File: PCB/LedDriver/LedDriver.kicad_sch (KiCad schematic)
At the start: 36 parts, among them J101 LCD, J102 Conn_01x07_Female, J103 Conn_01x02_Male, J104 Conn_01x02_Male, J105 Conn_01x02_Male, J106 Conn_01x02_Male, J107 DC+5V, J108 Conn_01x08_Male, J109 Conn_01x08_Male, J110 Conn_01x08_Male, J111 Conn_01x02_Male, SW101 SW_Push, SW102 SW_Push, SW103 SW_Push, SW104 SW_Push, SW105 SW_Push, SW106 SW_Push, SW107 SW_Push, U101 MW-R-WX, U102 LM1117-3.3, U103 LM35-LP

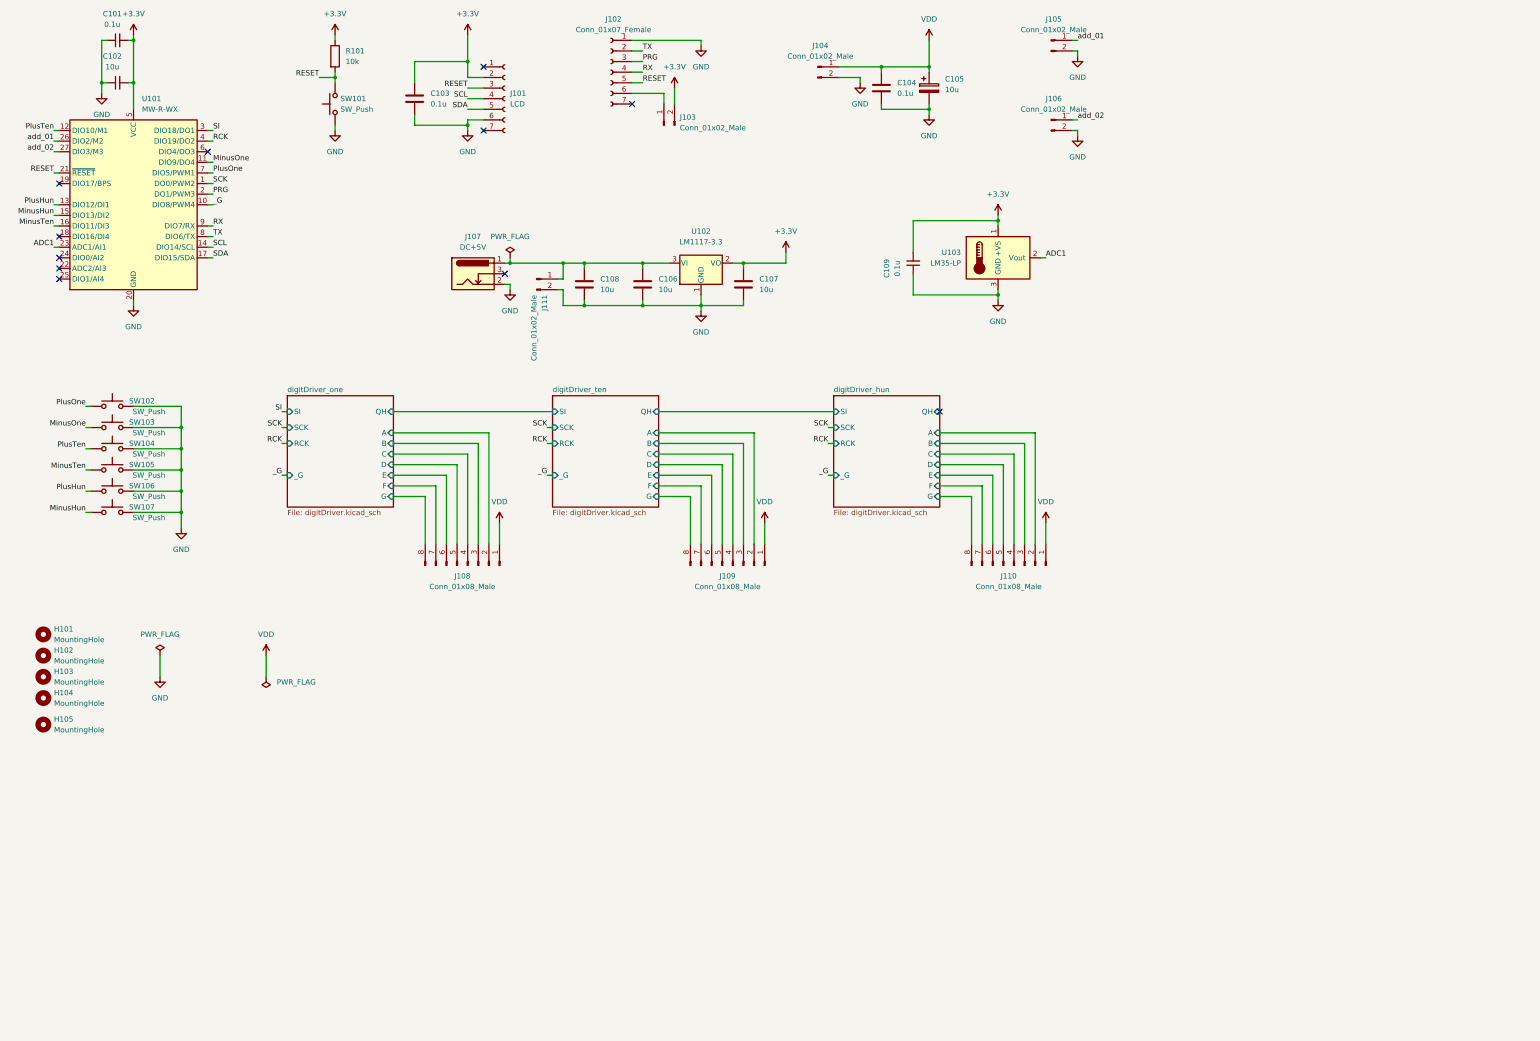
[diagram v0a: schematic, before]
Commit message: branch change
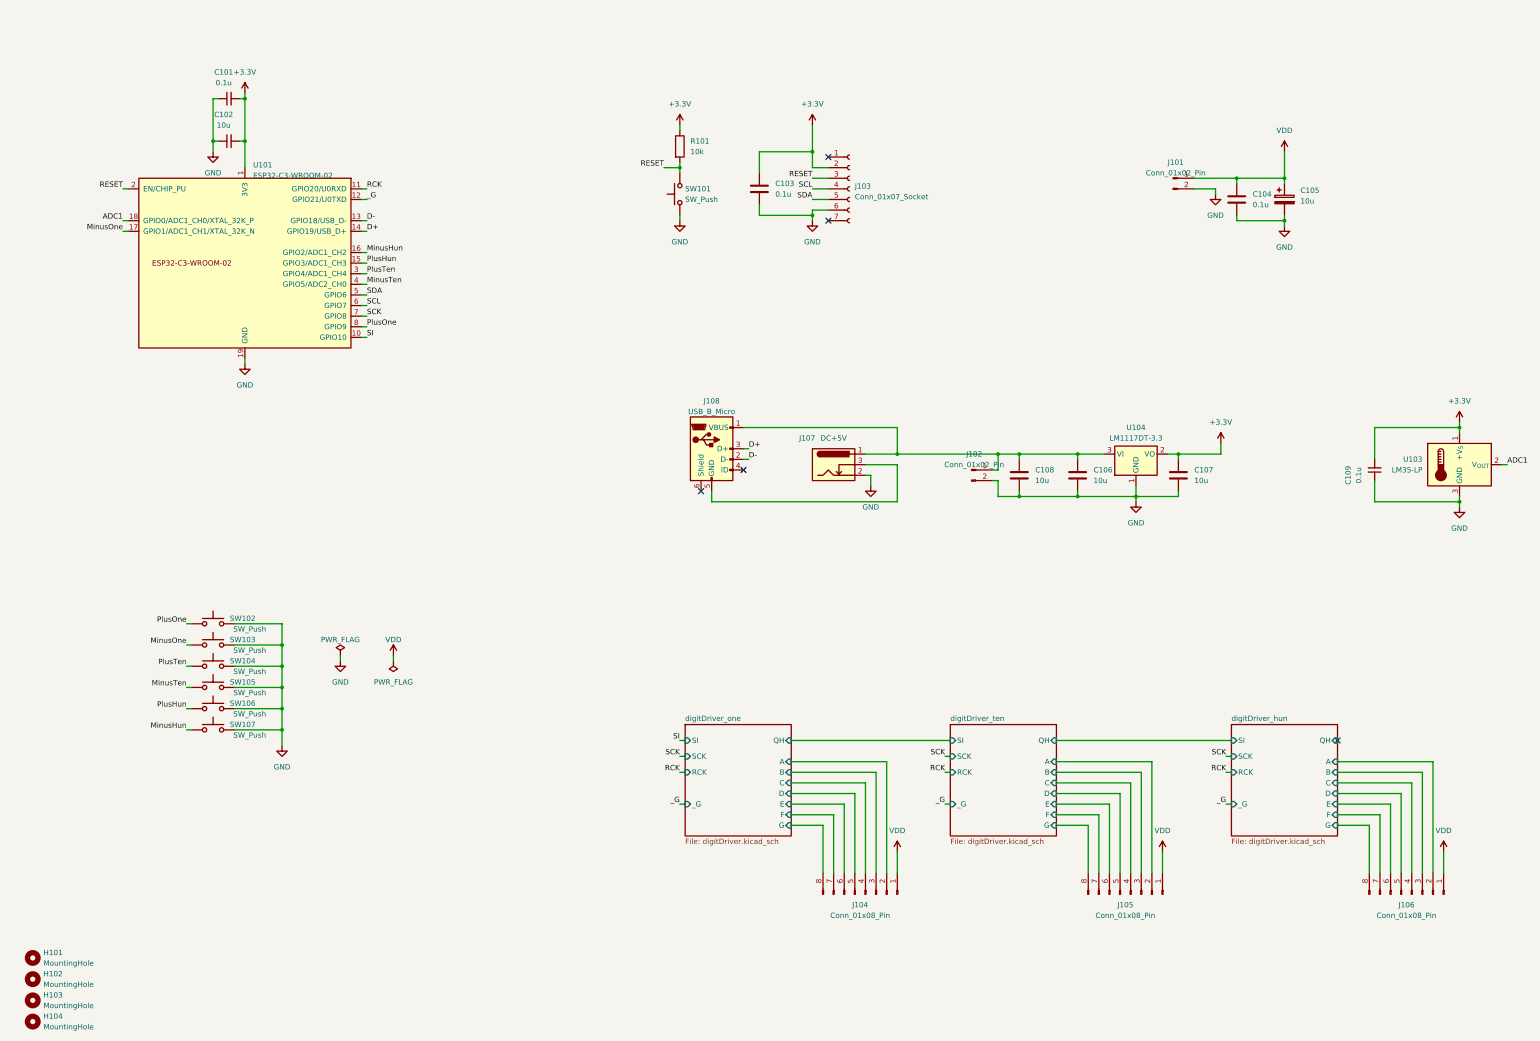
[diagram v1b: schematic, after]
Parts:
- removed H105: MountingHole, MountingHole:MountingHole_6.4mm_M6, symbol Mechanical:MountingHole
- removed J101: LCD, Connector_PinSocket_2.54mm:PinSocket_1x07_P2.54mm_Vertical, symbol Connector:Conn_01x07_Female
- removed J102: Conn_01x07_Female, Connector_PinSocket_2.54mm:PinSocket_1x07_P2.54mm_Vertical, symbol Connector:Conn_01x07_Female
- removed J103, J105, J106: Conn_01x02_Male, Connector_PinHeader_2.54mm:PinHeader_1x02_P2.54mm_Vertical, symbol Connector:Conn_01x02_Male
- removed J104: Conn_01x02_Male, Connector_JST:JST_VH_B2P-VH_1x02_P3.96mm_Vertical, symbol Connector:Conn_01x02_Male
- removed J108, J109, J110: Conn_01x08_Male, Connector_JST:JST_VH_B8P-VH_1x08_P3.96mm_Vertical, symbol Connector:Conn_01x08_Male
- removed J111: Conn_01x02_Male, Connector_JST:JST_XH_B2B-XH-A_1x02_P2.50mm_Vertical, symbol Connector:Conn_01x02_Male
- removed U101: MW-R-WX, RF_Module:MonoWireless_TWE-L-WX, symbol RF_ZigBee:MW-R-WX
- removed U102: LM1117-3.3, Package_TO_SOT_SMD:SOT-223-3_TabPin2, symbol Regulator_Linear:LM1117-3.3
- added J101: Conn_01x02_Pin, Connector_JST:JST_VH_B2P-VH_1x02_P3.96mm_Vertical, symbol Connector:Conn_01x02_Pin
- added J102: Conn_01x02_Pin, Connector_JST:JST_XH_B2B-XH-A_1x02_P2.50mm_Vertical, symbol Connector:Conn_01x02_Pin
- added J103: Conn_01x07_Socket, Connector_PinSocket_2.54mm:PinSocket_1x07_P2.54mm_Vertical, symbol Connector:Conn_01x07_Socket
- added J104, J105, J106: Conn_01x08_Pin, Connector_JST:JST_VH_B8P-VH_1x08_P3.96mm_Vertical, symbol Connector:Conn_01x08_Pin
- added J108: USB_B_Micro, footprints:ZX62R-B-5P30, symbol Connector:USB_B_Micro
- added U101: ESP32-C3-WROOM-02, Espressif:ESP32-C3-WROOM-02, symbol Espressif:ESP32-C3-WROOM-02
- added U104: LM1117DT-3.3, Package_TO_SOT_SMD:SOT-223-3_TabPin2, symbol Regulator_Linear:LM1117DT-3.3
- U103: footprint Package_TO_SOT_THT:TO-92_Inline_Horizontal1 -> Package_TO_SOT_THT:TO-92_Inline
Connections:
- net +3.3V: now also J103.2 (Pin_2), U101.1 (3V3), U104.2 (VO)
- net ADC1: now also U101.18 (GPIO0/ADC1_CH0/XTAL_32K_P)
- net GND: now also J101.2 (Pin_2), J102.2 (Pin_2), J103.6 (Pin_6), U101.19 (GND), U101.9 (GND), U104.1 (GND)
- net MinusHun: now also U101.16 (GPIO2/ADC1_CH2)
- net MinusOne: now also U101.17 (GPIO1/ADC1_CH1/XTAL_32K_N)
- net MinusTen: now also U101.4 (GPIO5/ADC2_CH0)
- net PlusHun: now also U101.15 (GPIO3/ADC1_CH3)
- net PlusOne: now also U101.8 (GPIO9)
- net PlusTen: now also U101.3 (GPIO4/ADC1_CH4)
- net RCK: now also U101.11 (GPIO20/U0RXD)
- net RESET: now also J103.3 (Pin_3), U101.2 (EN/CHIP_PU)
- net SCK: now also U101.7 (GPIO8)
- net SCL: now also J103.4 (Pin_4), U101.6 (GPIO7)
- net SDA: now also J103.5 (Pin_5), U101.5 (GPIO6)
- net SI: now also U101.10 (GPIO10)
- net VDD: now also J101.1 (Pin_1), J104.1 (Pin_1), J105.1 (Pin_1), J106.1 (Pin_1)
- net _G: now also U101.12 (GPIO21/U0TXD)
- net digitDriver_hun/A: now also J106.2 (Pin_2)
- net digitDriver_hun/B: now also J106.3 (Pin_3)
- net digitDriver_hun/C: now also J106.4 (Pin_4)
- net digitDriver_hun/D: now also J106.5 (Pin_5)
- net digitDriver_hun/E: now also J106.6 (Pin_6)
- net digitDriver_hun/F: now also J106.7 (Pin_7)
- net digitDriver_hun/G: now also J106.8 (Pin_8)
- net digitDriver_one/A: now also J104.2 (Pin_2)
- net digitDriver_one/B: now also J104.3 (Pin_3)
- net digitDriver_one/C: now also J104.4 (Pin_4)
- net digitDriver_one/D: now also J104.5 (Pin_5)
- net digitDriver_one/E: now also J104.6 (Pin_6)
- net digitDriver_one/F: now also J104.7 (Pin_7)
- net digitDriver_one/G: now also J104.8 (Pin_8)
- net digitDriver_ten/A: now also J105.2 (Pin_2)
- net digitDriver_ten/B: now also J105.3 (Pin_3)
- net digitDriver_ten/C: now also J105.4 (Pin_4)
- net digitDriver_ten/D: now also J105.5 (Pin_5)
- net digitDriver_ten/E: now also J105.6 (Pin_6)
- net digitDriver_ten/F: now also J105.7 (Pin_7)
- net digitDriver_ten/G: now also J105.8 (Pin_8)
- net at C106.1, C108.1, J107.1: now also J102.1 (Pin_1), J108.1 (VBUS), U104.3 (VI)
- net at J107.3: now also J108.5 (GND)
- new net D+: J108.3 (D+), U101.14 (GPIO19/USB_D+)
- new net D-: J108.2 (D-), U101.13 (GPIO18/USB_D-)
- no-connect marks 11 -> 5
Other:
- moved on the sheet: C101, C102, C103, C104, C105, C106, C107, C108, C109, H101, H102, H103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
